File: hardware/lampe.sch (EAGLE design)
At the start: 30 parts, among them IC1 ATMEGA168-20P, IC3 DS1307, Q2 16Mhz, Q3 32.768kHz, Q4 BUZ11BV, T3 BC547B, T4 BC547B, X1 MKDSN1,5/2-5,08, X2 MKDSN1,5/2-5,08

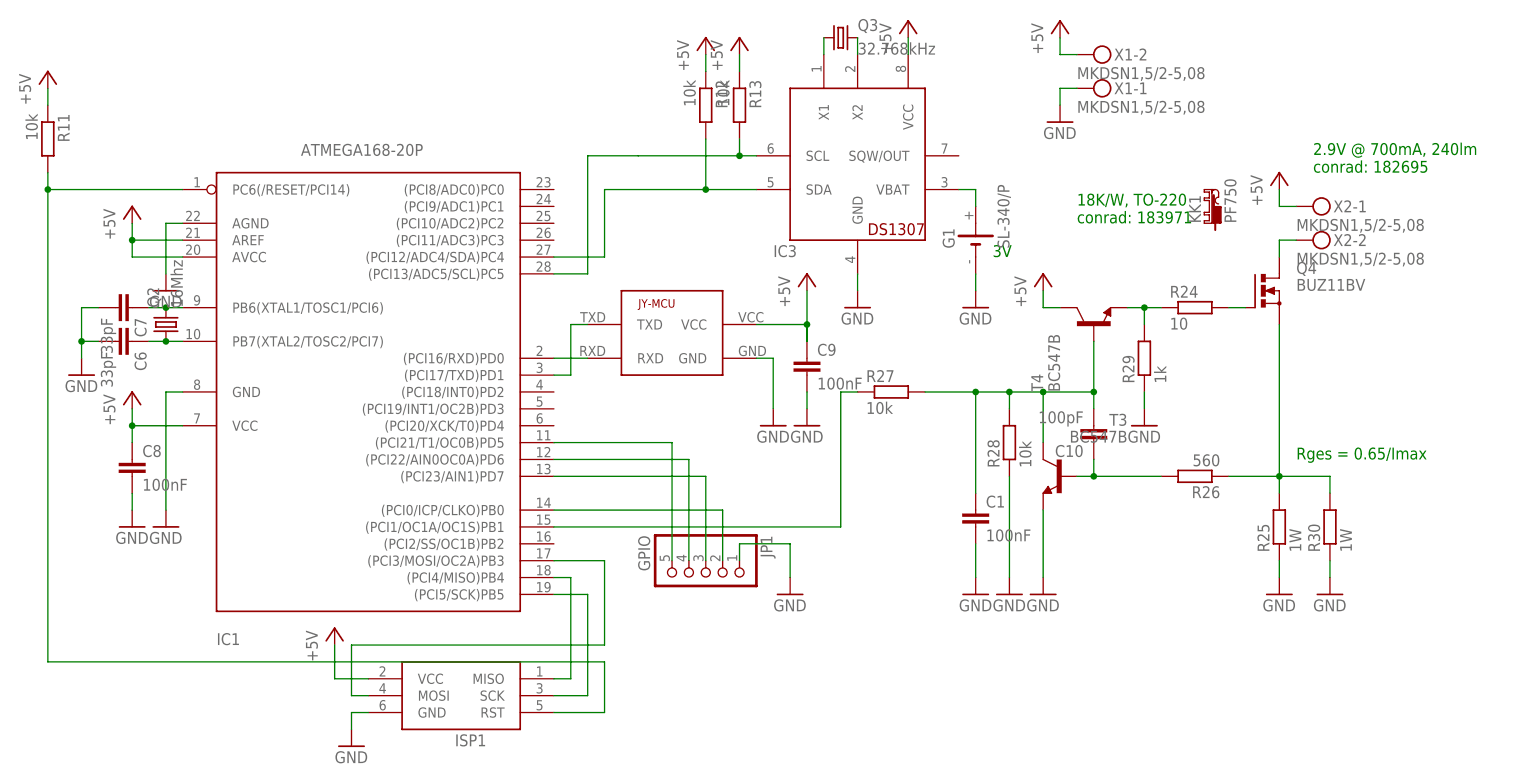
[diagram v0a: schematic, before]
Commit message: Minors.
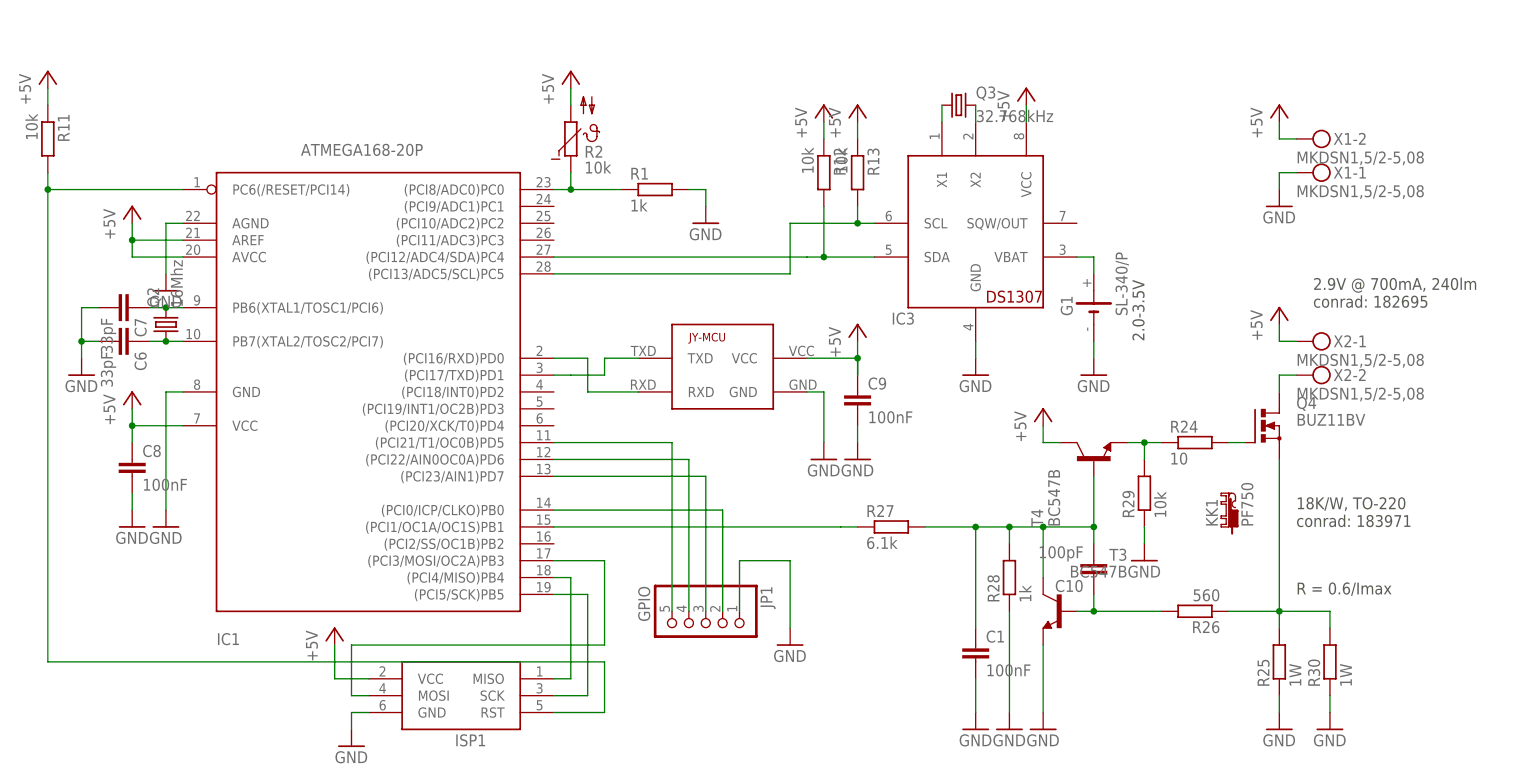
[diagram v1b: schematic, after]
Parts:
- added R1: 1k, rcl:R-EU_0204/2V
- added R2: 10k, ptc-ntc:B57164
- R27: value 10k -> 6.1k
- R28: value 10k -> 1k
- R29: value 1k -> 10k
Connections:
- new net N$10: IC1.(PCI8/ADC0)PC0, R1.1, R2.1
- net +5V: now also R2.2
- net GND: now also R1.2
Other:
- note added: "2.0-3.5V"
- note added: "R = 0.6/Imax"
- note removed: "3V"
- note removed: "Rges = 0.65/Imax"
- moved on the sheet: C1, C10, C9, G1, IC3, JP1, KK1, Q3, Q4, R12, R13, R24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
